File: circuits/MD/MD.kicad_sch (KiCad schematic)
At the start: 45 parts, among them J2 Conn_01x10_Male, J7 Conn_01x06_MountingPin, J8 Conn_01x06_MountingPin, Q10 S8050, Q11 S8050, SW2 SW_SPST, SW3 SW_SPST, SW5 SW_DIP_x02, U2 STM32G473CET6, U5 STM32F446RETx, U6 MAX3485, U7 MAX3485, Y1 16MHz, Y2 32.768kHz

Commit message: こみっと
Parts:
- removed C22, C34, C35, C36, C37, C38, C39: 0.1uF, Capacitor_SMD:C_0402_1005Metric, symbol Device:C
- removed C24, C31, C33: 22pF, Capacitor_SMD:C_0603_1608Metric, symbol Device:C
- removed J2: Conn_01x10_Male, MyLibrary:BoxHeader_2x05_P1.27mm_Vertical_SMD, symbol Connector:Conn_01x10_Male
- removed J7, J8: Conn_01x06_MountingPin, Connector_Molex:Molex_PicoBlade_53261-0671_1x06-1MP_P1.25mm_Horizontal, symbol Connector_Generic_MountingPin:Conn_01x06_MountingPin
- removed JP1, JP2: Jumper_2_Open, Connector_PinHeader_2.54mm:PinHeader_1x02_P2.54mm_Vertical, symbol Jumper:Jumper_2_Open
- removed Q10, Q11: S8050, Package_TO_SOT_SMD:SOT-23, symbol Device:Q_PNP_BEC
- removed R61, R69, R70: 10k, Resistor_SMD:R_0402_1005Metric, symbol Device:R
- removed R65, R72: 20k, Resistor_SMD:R_0402_1005Metric, symbol Device:R
- removed R66, R67, R73, R74: 2.2k, Resistor_SMD:R_0402_1005Metric, symbol Device:R
- removed R68, R75: 120, Resistor_SMD:R_0402_1005Metric, symbol Device:R
- removed R71: 7.5k, Resistor_SMD:R_0603_1608Metric, symbol Device:R
- removed SW2, SW3: SW_SPST, Button_Switch_SMD:SW_Push_1P1T_NO_Vertical_Wuerth_434133025816, symbol Switch:SW_SPST
- removed SW5: SW_DIP_x02, Package_DIP:DIP-4_W7.62mm, symbol Switch:SW_DIP_x02
- removed U6, U7: MAX3485, Package_SO:SOP-8_3.9x4.9mm_P1.27mm, symbol Interface_UART:MAX3485
- removed Y1: 16MHz, Crystal:Crystal_SMD_3225-4Pin_3.2x2.5mm_HandSoldering, symbol Device:Crystal_GND24
- removed Y2: 32.768kHz, Crystal:Crystal_SMD_3215-2Pin_3.2x1.5mm, symbol Device:Crystal
- added C44, C45: 22pF, Capacitor_SMD:C_0603_1608Metric, symbol Device:C
- added C46, C48, C50, C51, C52, C53: 0.1uF, Capacitor_SMD:C_0402_1005Metric, symbol Device:C
- added D22: 1N5819WS, Diode_SMD:D_SOD-323_HandSoldering, symbol Device:D_Schottky
- added J3: Conn_01x14_Pin, symbol Connector:Conn_01x14_Pin
- added R79: 1k, Resistor_SMD:R_0402_1005Metric, symbol Device:R
- added SW4, SW6: SW_SPST, Button_Switch_SMD:SW_Push_1P1T_NO_Vertical_Wuerth_434133025816, symbol Switch:SW_SPST
- added Y3: 16MHz, Crystal:Crystal_SMD_3225-4Pin_3.2x2.5mm_HandSoldering, symbol Device:Crystal_GND24
- added Y4: 32.768kHz, Crystal:Crystal_SMD_3215-2Pin_3.2x1.5mm, symbol Device:Crystal
- C32: value 22pF -> 1uF; footprint Capacitor_SMD:C_0603_1608Metric -> Capacitor_SMD:C_0402_1005Metric
- C42, C43: value 0.1uF -> 22pF; footprint Capacitor_SMD:C_0402_1005Metric -> Capacitor_SMD:C_0603_1608Metric
- R64: value 7.5k -> 10k; footprint Resistor_SMD:R_0603_1608Metric -> Resistor_SMD:R_0402_1005Metric
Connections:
- net +3.3V: now also C32.1, U2.1 (VBAT), U2.20 (VREF+), U2.21 (VDDA), U2.24 (VDD), U2.36 (VDD), U2.48 (VDD), C46.1, C48.1, C50.1, C52.1, C53.1, D22.2 (A), SW4.2 (B); no longer C42.1, C43.1
- net BOOT0: now also R64.1, SW4.1 (A)
- net GND: no longer C32.1, C42.2, C43.2
- net GNDD: now also C32.2, C42.1, C43.1, R64.2, U2.19 (VSSA), U2.23 (VSS), U2.35 (VSS), U2.47 (VSS), C44.1, C45.1, C46.2, C48.2, C50.2, C51.2, C52.2, C53.2, J3.11 (Pin_11), J3.5 (Pin_5), J3.7 (Pin_7), R79.2, SW6.2 (B), Y3.2, Y3.4
- net HSE_IN: now also C42.2, Y3.1
- net HSE_OUT: now also C43.2, Y3.3
- net LSE_IN: now also C44.2, Y4.2; no longer C32.2
- net LSE_OUT: now also C45.2, Y4.1
- net MainTX6_RS485aRX: no longer R64.2
- net NRST: now also C51.1, J3.12 (Pin_12), SW6.1 (A)
- net SWO: now also J3.8 (Pin_8)
- new net: D22.1 (K), J3.3 (Pin_3), R79.1
- new net SWCLK: J3.6 (Pin_6)
- new net SWDIO: J3.4 (Pin_4)
- no-connect marks 2 -> 6
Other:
- added sheet Encoder (Encoder.kicad_sch)
- added sheet RS485 (RS485.kicad_sch)
- added sheet UI (UI.kicad_sch)
- sheet Power ports: added V_Meas.; removed V_Measure
- note added: "G473CE"
- note added: "マイコンなどの起動管理システム ダイオードなど耐圧確認 BOOTのプルダウンとかなんだとか SWDピンのリセット時の挙動だとか G473のデータシートを見る VREF,VBATについて"
- note added: "書き込み"
- note removed: "Conn"
- note removed: "MAX3485"
- note removed: "RS485a"
- note removed: "マイコンなどの起動管理システム ダイオードなど耐圧確認"
- moved on the sheet: C40, C41, R63, U2, U5

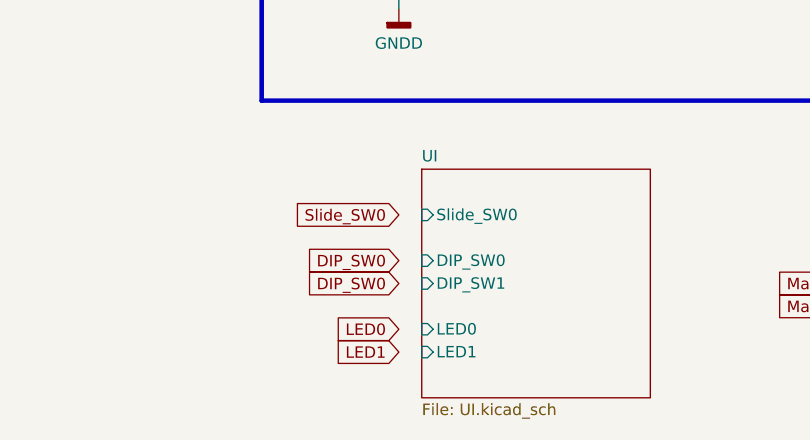
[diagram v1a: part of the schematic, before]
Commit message: とちゅう
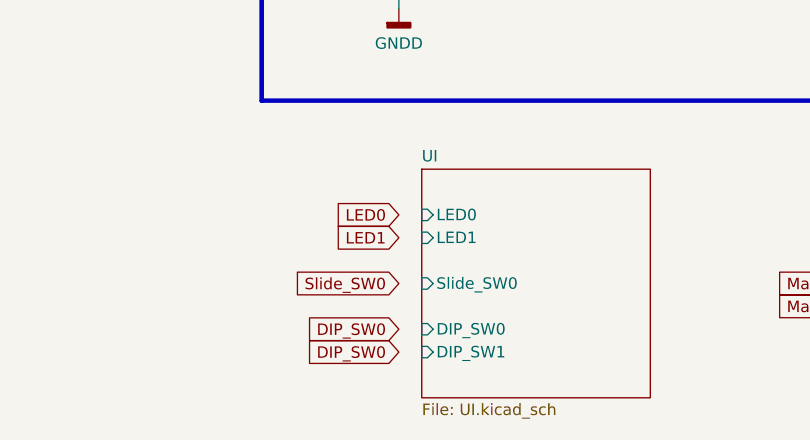
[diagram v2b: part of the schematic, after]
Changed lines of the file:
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@@
     (stroke (width 0) (type default))
   )
-  (wire (pts (xy 114.3 177.8) (xy 116.84 177.8))
+  (wire (pts (xy 114.3 175.26) (xy 116.84 175.26))
     (stroke (width 0) (type default))
   )
@@
     (stroke (width 0) (type default))
   )
-  (wire (pts (xy 114.3 175.26) (xy 116.84 175.26))
+  (wire (pts (xy 114.3 177.8) (xy 116.84 177.8))
     (stroke (width 0) (type default))
   )
@@
     )
   )
-  (global_label "LED0" (shape input) (at 53.34 180.34 180) (fields_autoplaced)
-    (effects (font (size 1.27 1.27)) (justify right))
-    (property "Intersheetrefs" "${INTERSHEET_REFS}" (at 45.6982 180.34 0)
+  (global_label "LED0" (shape input) (at 53.34 167.64 180) (fields_autoplaced)
+    (effects (font (size 1.27 1.27)) (justify right))
+    (property "Intersheetrefs" "${INTERSHEET_REFS}" (at 45.6982 167.64 0)
       (effects (font (size 1.27 1.27)) (justify right) hide)
     )
@@
     )
   )
-  (global_label "DIP_SW0" (shape input) (at 53.34 172.72 180) (fields_autoplaced)
-    (effects (font (size 1.27 1.27)) (justify right))
-    (property "Intersheetrefs" "${INTERSHEET_REFS}" (at 42.372 172.72 0)
+  (global_label "DIP_SW0" (shape input) (at 53.34 180.34 180) (fields_autoplaced)
+    (effects (font (size 1.27 1.27)) (justify right))
+    (property "Intersheetrefs" "${INTERSHEET_REFS}" (at 42.372 180.34 0)
       (effects (font (size 1.27 1.27)) (justify right) hide)
     )
@@
     )
   )
-  (global_label "LED1" (shape input) (at 53.34 182.88 180) (fields_autoplaced)
-    (effects (font (size 1.27 1.27)) (justify right))
-    (property "Intersheetrefs" "${INTERSHEET_REFS}" (at 45.6982 182.88 0)
+  (global_label "LED1" (shape input) (at 53.34 170.18 180) (fields_autoplaced)
+    (effects (font (size 1.27 1.27)) (justify right))
+    (property "Intersheetrefs" "${INTERSHEET_REFS}" (at 45.6982 170.18 0)
       (effects (font (size 1.27 1.27)) (justify right) hide)
     )
@@
     )
   )
-  (global_label "Slide_SW0" (shape input) (at 53.34 167.64 180) (fields_autoplaced)
-    (effects (font (size 1.27 1.27)) (justify right))
-    (property "Intersheetrefs" "${INTERSHEET_REFS}" (at 40.7997 167.64 0)
+  (global_label "Slide_SW0" (shape input) (at 53.34 175.26 180) (fields_autoplaced)
+    (effects (font (size 1.27 1.27)) (justify right))
+    (property "Intersheetrefs" "${INTERSHEET_REFS}" (at 40.7997 175.26 0)
       (effects (font (size 1.27 1.27)) (justify right) hide)
     )
@@
     )
   )
-  (global_label "DIP_SW0" (shape input) (at 53.34 175.26 180) (fields_autoplaced)
-    (effects (font (size 1.27 1.27)) (justify right))
-    (property "Intersheetrefs" "${INTERSHEET_REFS}" (at 42.372 175.26 0)
+  (global_label "DIP_SW0" (shape input) (at 53.34 182.88 180) (fields_autoplaced)
+    (effects (font (size 1.27 1.27)) (justify right))
+    (property "Intersheetrefs" "${INTERSHEET_REFS}" (at 42.372 182.88 0)
       (effects (font (size 1.27 1.27)) (justify right) hide)
     )
@@
       (effects (font (size 1.27 1.27)) (justify left top))
     )
-    (pin "LED0" input (at 55.88 180.34 180)
-      (effects (font (size 1.27 1.27)) (justify left))
-    )
-    (pin "LED1" input (at 55.88 182.88 180)
-      (effects (font (size 1.27 1.27)) (justify left))
-    )
-    (pin "Slide_SW0" input (at 55.88 167.64 180)
-      (effects (font (size 1.27 1.27)) (justify left))
-    )
-    (pin "DIP_SW1" input (at 55.88 175.26 180)
-      (effects (font (size 1.27 1.27)) (justify left))
-    )
-    (pin "DIP_SW0" input (at 55.88 172.72 180)
-      (effects (font (size 1.27 1.27)) (justify left))
-    )
+    (pin "LED0" input (at 55.88 167.64 180)
+      (effects (font (size 1.27 1.27)) (justify left))
+    )
+    (pin "LED1" input (at 55.88 170.18 180)
+      (effects (font (size 1.27 1.27)) (justify left))
+    )
+    (pin "Slide_SW0" input (at 55.88 175.26 180)
+      (effects (font (size 1.27 1.27)) (justify left))
+    )
+    (pin "DIP_SW1" input (at 55.88 182.88 180)
+      (effects (font (size 1.27 1.27)) (justify left))
+    )
+    (pin "DIP_SW0" input (at 55.88 180.34 180)
+      (effects (font (size 1.27 1.27)) (justify left))
+    )

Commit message: すてい
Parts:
- removed C32, C41: 1uF, Capacitor_SMD:C_0402_1005Metric, symbol Device:C
- removed C40: 4.7uF, Capacitor_SMD:C_0603_1608Metric, symbol Device:C
- removed C44, C45: 22pF, Capacitor_SMD:C_0603_1608Metric, symbol Device:C
- removed R63: 10k, Resistor_SMD:R_0402_1005Metric, symbol Device:R
- removed SW4: SW_SPST, Button_Switch_SMD:SW_Push_1P1T_NO_Vertical_Wuerth_434133025816, symbol Switch:SW_SPST
- removed U5: STM32F446RETx, symbol MCU_ST_STM32F4:STM32F446RETx
- removed Y4: 32.768kHz, Crystal:Crystal_SMD_3215-2Pin_3.2x1.5mm, symbol Device:Crystal
- added C22: 4.7uF, Capacitor_SMD:C_0603_1608Metric, symbol Device:C
- added R55: 10k, Resistor_SMD:R_0402_1005Metric, symbol Device:R
- J3: footprint (none) -> MyLibrary:BoxHeader_2x07_P1.27mm_Horizontal
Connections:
- net +3.3V: now also C22.2
- net BOOT0: now also U2.45 (PB8-BOOT0)
- net Current_OUTA: now also U2.8 (PA0)
- net Current_OUTB: now also U2.9 (PA1)
- net Current_OUTC: now also U2.10 (PA2)
- net GNDD: now also C22.1, R55.2
- net HSE_IN: now also U2.5 (PF0)
- net HSE_OUT: now also U2.6 (PF1)
- net MainRX3_RS485TX: now also U2.25 (PB11)
- net MainTX3_RS485RX: now also U2.22 (PB10)
- net NRST: now also U2.7 (NRST)
- net SWCLK: now also U2.38 (PA14)
- net SWDIO: now also U2.37 (PA13)
- net SWO: now also U2.40 (PB3)
- net V_Meas.: now also U2.11 (PA3)
- net SCLK1: now reaches U2.13 (PA5)
- net MISO1: now reaches U2.14 (PA6)
- net MOSI1: now reaches U2.15 (PA7)
- net at U2.18 (PB2): now also R55.1
- no-connect marks 6 -> 11
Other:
- note added: "マイコンなどの起動管理システム ダイオードなど耐圧確認 BOOTのプルダウンとかなんだとか SWDピンのリセット時の挙動だとか G473のデータシートを見る"
- note removed: "F446RE"
- note removed: "LSE"
- note removed: "マイコンなどの起動管理システム ダイオードなど耐圧確認 BOOTのプルダウンとかなんだとか SWDピンのリセット時の挙動だとか G473のデータシートを見る VREF,VBATについて"
- moved on the sheet: C42, C43, C46, C48, C50, C51, C52, C53, D22, J3, R64, R79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
